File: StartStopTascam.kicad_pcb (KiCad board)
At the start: 2 copper layers, 69.1 x 53.8 mm, 19 parts, among them J1 Jack_Stack_LJB0671, J2 Jack_Stack_LJB0671, J3 DB9_Male, P1 CONN_02X03, U1 MAX232

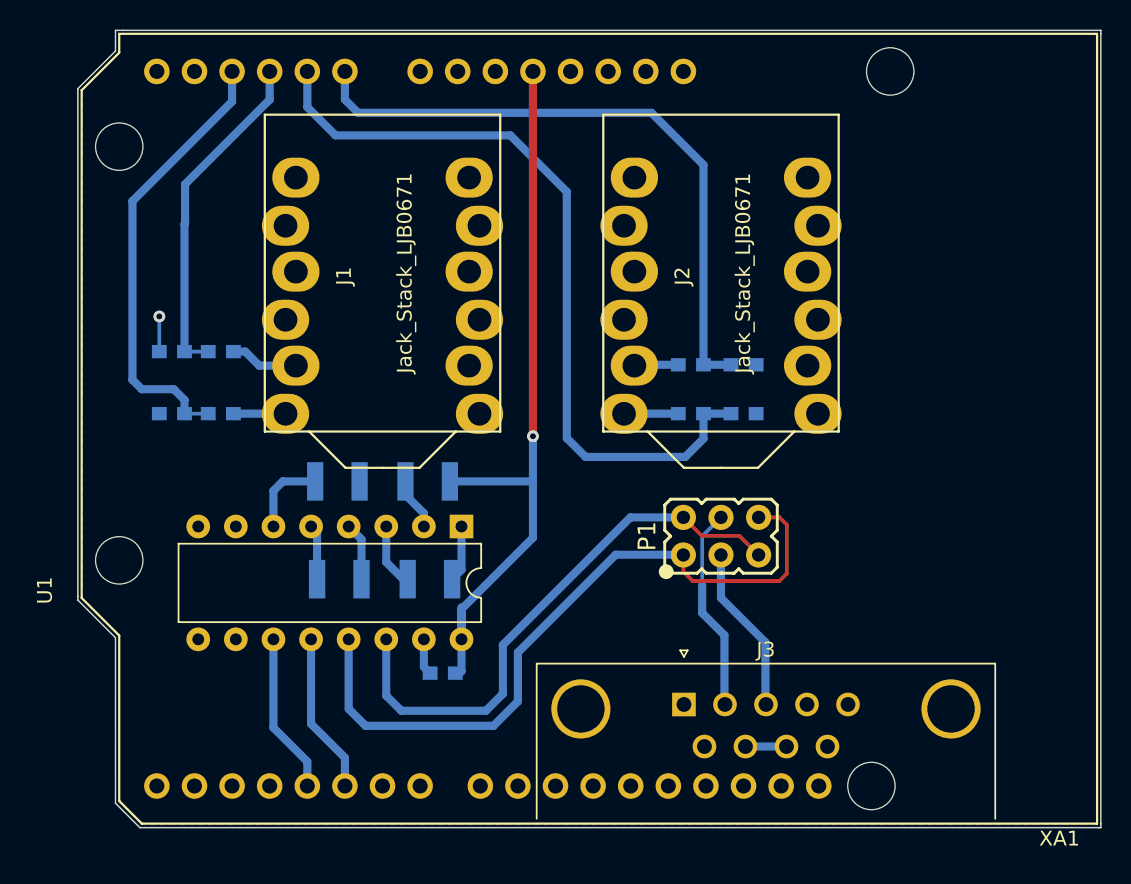
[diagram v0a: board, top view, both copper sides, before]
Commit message: kicad
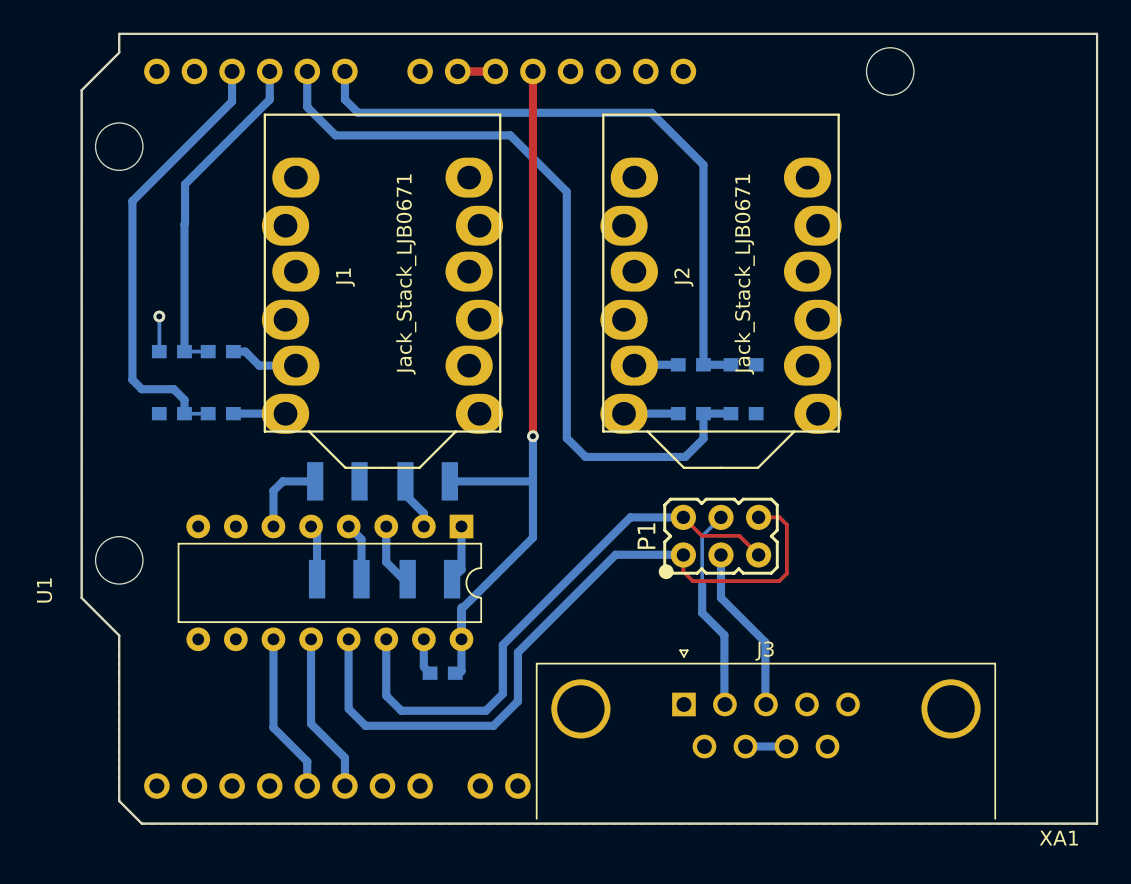
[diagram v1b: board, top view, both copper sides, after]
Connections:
- XA1 pad GND2: unconnected-(XA1-PadGND2) -> /GND
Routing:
- net /GND: track 4.89 -> 7.43 mm
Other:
- board size 69.1 x 53.8 mm -> 68.6 x 53.3 mm
